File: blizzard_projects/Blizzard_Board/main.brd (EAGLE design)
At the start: 80 x 80 mm, 84 parts, among them J1 XH_4POS_DEV, J2 XH_5POS_DEV, J3 XH_4POS_DEV, J4 XH_6POS_DEV, J5 XH_5POS_DEV, J6 XH_2POS_DEV, J7 XH_2POS_DEV, Q1 s8050(NPN), Q2 S8050(NPN), Q3 N2222, Q4 N2222, U1 USB_TO_UART_DEV, U2 BUCK_CONVERTER_DEV, U3 ESP_WROOM_32_DEV, U4 LAN8720_DEV, U5 MAX_485_DEV, X1 USB_CONN_DEV, X2 ETHERNET_DEV, Y1 50MHz

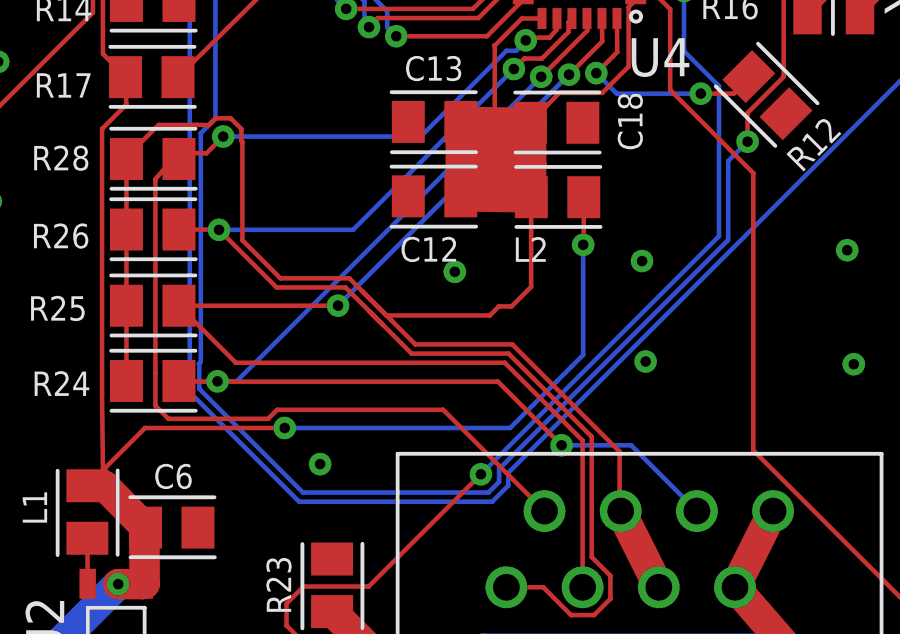
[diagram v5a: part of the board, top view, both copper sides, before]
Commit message: REV 1.2
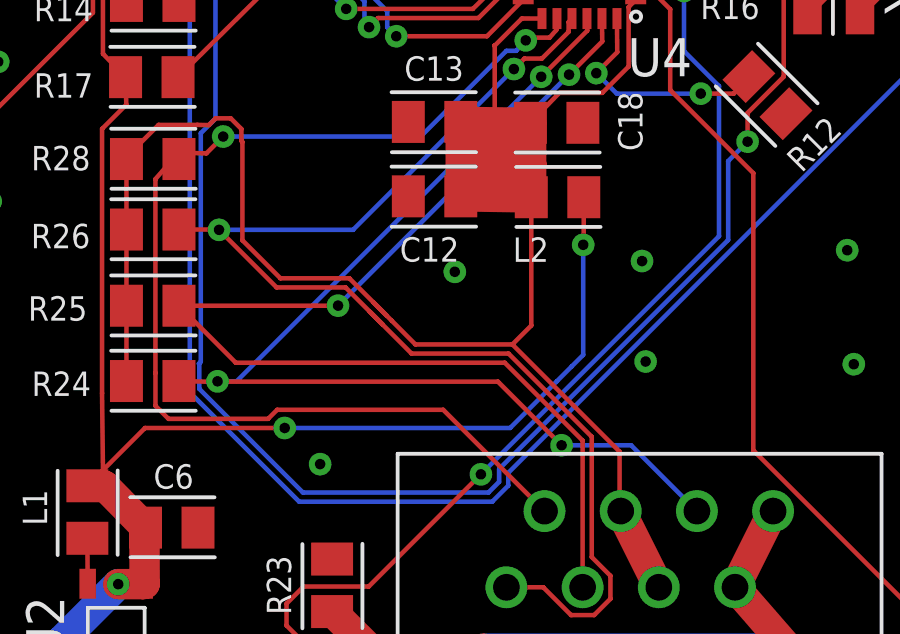
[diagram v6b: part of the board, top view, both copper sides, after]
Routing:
- net ETH_VDD: track 77.0 -> 72.9 mm
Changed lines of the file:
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@@
 <wire x1="33.989903125" y1="30.287" x2="33.985" y2="30.47354375" width="1.016" layer="1"/>
 <wire x1="33.985" y1="30.47354375" x2="32.545" y2="31.91354375" width="1.016" layer="1"/>
-<wire x1="33.985" y1="27.299228125" x2="33.985" y2="30.78488125" width="0.1524" layer="1"/>
 <wire x1="21.5653125" y1="32.6986" x2="22.8546875" y2="32.6986" width="0.1524" layer="1"/>
 <wire x1="23.46865" y1="32.9168" x2="23.97135" y2="32.9168" width="0.1524" layer="1"/>
@@
 <wire x1="24.36" y1="32.13" x2="24.36" y2="28.85105625" width="0.1524" layer="1"/>
 <wire x1="24.36" y1="28.85105625" x2="25.62685625" y2="27.5842" width="0.1524" layer="1"/>
-<wire x1="25.62685625" y1="27.5842" x2="27.92501875" y2="27.5842" width="0.1524" layer="1"/>
-<wire x1="28.3607375" y1="27.14848125" x2="27.92501875" y2="27.5842" width="0.1524" layer="1"/>
-<wire x1="28.3607375" y1="27.14848125" x2="29.16441875" y2="26.3448" width="0.1524" layer="1"/>
-<wire x1="29.16441875" y1="26.3448" x2="32.60665" y2="26.3448" width="0.1524" layer="1"/>
-<wire x1="32.60665" y1="26.3448" x2="32.90865" y2="26.6468" width="0.1524" layer="1"/>
-<wire x1="32.90865" y1="26.6468" x2="33.332571875" y2="26.6468" width="0.1524" layer="1"/>
-<wire x1="33.332571875" y1="26.6468" x2="33.985" y2="27.299228125" width="0.1524" layer="1"/>
+<wire x1="27.92501875" y1="27.5842" x2="25.62685625" y2="27.5842" width="0.1524" layer="1"/>
+<wire x1="28.736059375" y1="26.773159375" x2="27.92501875" y2="27.5842" width="0.1524" layer="1"/>
+<wire x1="28.736059375" y1="26.773159375" x2="29.16441875" y2="26.3448" width="0.1524" layer="1"/>
 <wire x1="20.494903125" y1="24.16" x2="20.494903125" y2="26.67" width="0.1524" layer="1"/>
 <wire x1="20.494903125" y1="26.67" x2="20.494903125" y2="29.21" width="0.1524" layer="1"/>
@@
 <wire x1="28.7362875" y1="26.773159375" x2="28.736059375" y2="26.773159375" width="0.1524" layer="1"/>
 <wire x1="29.3429625" y1="26.16625625" x2="28.824634375" y2="26.684584375" width="0.1524" layer="1"/>
-<wire x1="28.736059375" y1="26.773159375" x2="28.3607375" y2="27.14848125" width="0.1524" layer="1"/>
 <wire x1="30.127578125" y1="25.3796125" x2="29.3429625" y2="26.16625625" width="0.1524" layer="1"/>
-<wire x1="36.932409375" y1="21.805396875" x2="33.35819375" y2="25.3796125" width="0.1524" layer="1"/>
+<wire x1="33.35819375" y1="25.3796125" x2="36.932409375" y2="21.805396875" width="0.1524" layer="1"/>
 <wire x1="33.35819375" y1="25.3796125" x2="30.127578125" y2="25.3796125" width="0.1524" layer="1"/>
 <wire x1="36.97" y1="19.825" x2="36.932409375" y2="19.862590625" width="0.1524" layer="1"/>
 <wire x1="36.932409375" y1="19.862590625" x2="36.932409375" y2="21.805396875" width="0.1524" layer="1"/>
+<wire x1="33.989903125" y1="30.287" x2="33.989903125" y2="26.011321875" width="0.1524" layer="1"/>
+<wire x1="33.989903125" y1="26.011321875" x2="33.35819375" y2="25.3796125" width="0.1524" layer="1"/>
 </signal>
 <signal name="N$32">
